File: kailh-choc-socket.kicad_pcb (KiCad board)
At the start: 2 copper layers, 18 x 17 mm, 8 parts, among them SW1 SW_DIP_x01

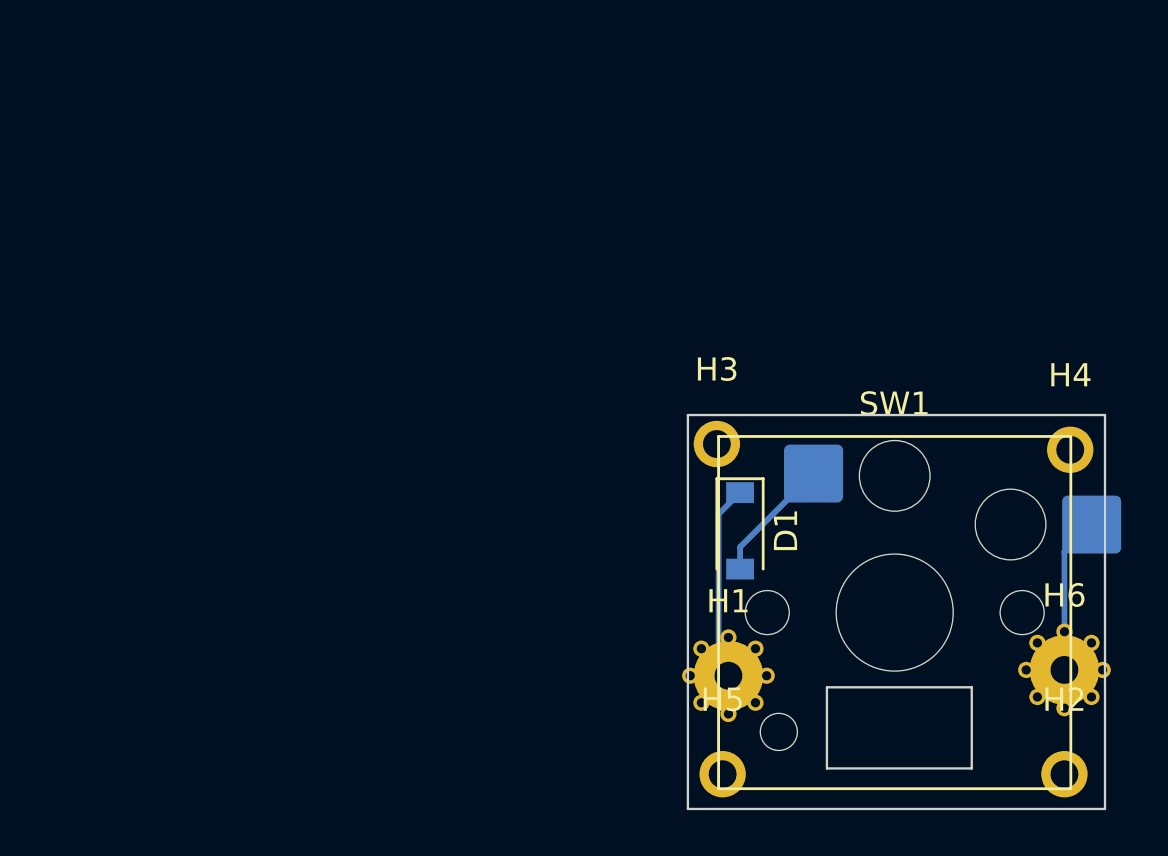
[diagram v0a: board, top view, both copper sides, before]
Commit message: Added layer details
M  .gitignore
M  README.md
M  fp-lib-table
M  kailh-choc-socket.kicad_pcb
M  kailh-choc-socket.kicad_prl
M  kailh-choc-socket.kicad_pro
M  kailh-choc-socket.kicad_sch
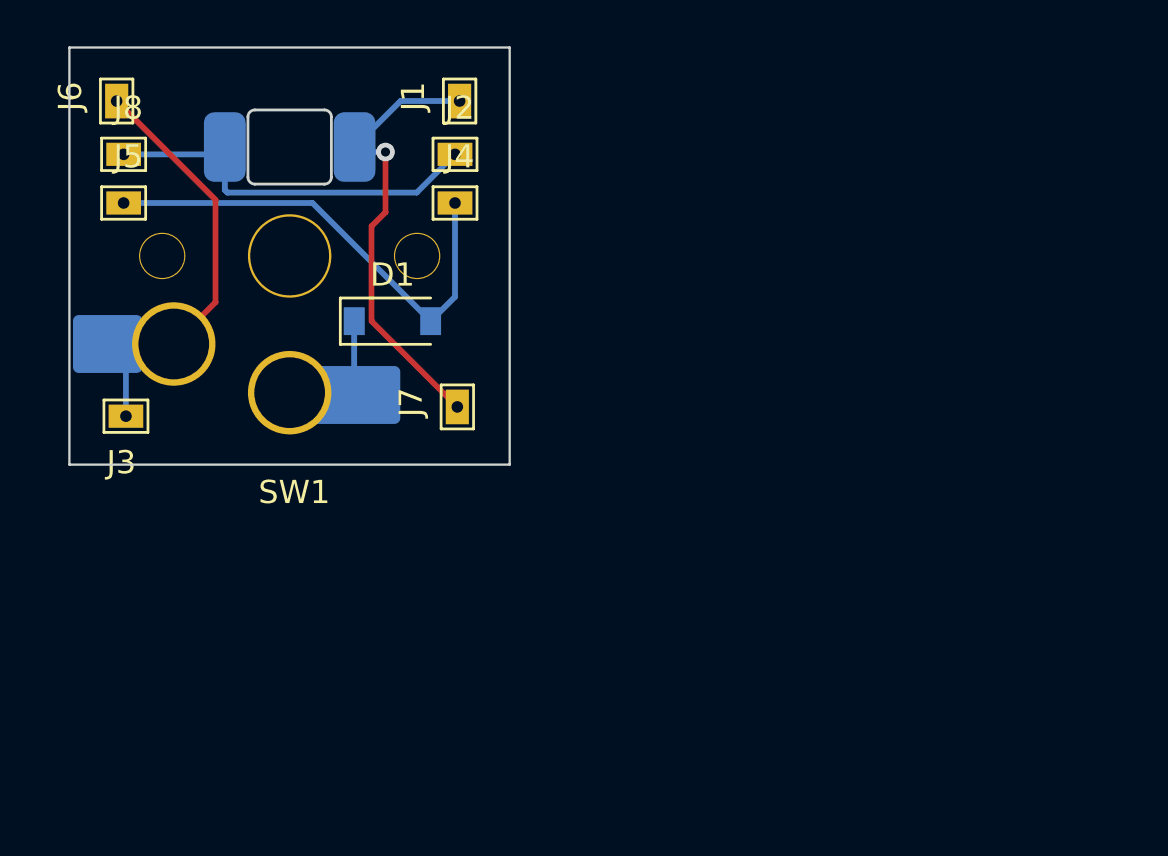
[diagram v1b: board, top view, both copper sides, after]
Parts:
- removed H1, H6: MountingHole_Pad, MountingHole:MountingHole_2.2mm_M2_Pad_Via
- removed H2, H3, H4, H5: MountingHole, MountingHole:MountingHole_2mm
- added J1: Conn_01x01_Male, Giri-Kailh-Choc-Library:TestPoint_THTPad_1.0x1.5mm_Drill0.5mm, F.Cu at (126.4, 69.2)
- added J2: Conn_01x01_Male, Giri-Kailh-Choc-Library:TestPoint_THTPad_1.0x1.5mm_Drill0.5mm, F.Cu at (126.2, 71.5)
- added J3: Conn_01x01_Male, Giri-Kailh-Choc-Library:TestPoint_THTPad_1.0x1.5mm_Drill0.5mm, F.Cu at (112.0, 82.8)
- added J4: Conn_01x01_Male, Giri-Kailh-Choc-Library:TestPoint_THTPad_1.0x1.5mm_Drill0.5mm, F.Cu at (126.2, 73.6)
- added J5: Conn_01x01_Male, Giri-Kailh-Choc-Library:TestPoint_THTPad_1.0x1.5mm_Drill0.5mm, F.Cu at (111.9, 73.6)
- added J6: Conn_01x01_Male, Giri-Kailh-Choc-Library:TestPoint_THTPad_1.0x1.5mm_Drill0.5mm, F.Cu at (111.6, 69.2)
- added J7: Conn_01x01_Male, Giri-Kailh-Choc-Library:TestPoint_THTPad_1.0x1.5mm_Drill0.5mm, F.Cu at (126.3, 82.4)
- added J8: Conn_01x01_Male, Giri-Kailh-Choc-Library:TestPoint_THTPad_1.0x1.5mm_Drill0.5mm, F.Cu at (111.9, 71.5)
- SW1: value SW_DIP_x01 -> SW_DIP_x02; footprint Switch_Keyboard_Hotswap_Kailh:SW_Hotswap_Kailh_Choc_V1_1.00u -> Giri-Kailh-Choc-Library:SW_Hotswap_Kailh_Choc_V1_plated_girish2
- moved SW1 30.3 mm to (119.1, 75.9)
- moved D1 17.5 mm to (123.5, 78.7), turned to 0 degrees
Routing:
- net Net-(J6-Pad1): track 0.00 -> 17.4 mm
- net Net-(J2-Pad1): track 0.00 -> 17.0 mm
- net Net-(J1-Pad1): track 6.76 -> 19.6 mm, vias 0 -> 1
- net Net-(J4-Pad1): track 8.46 -> 20.9 mm
- net Net-(D1-Pad1): track 5.44 -> 3.21 mm
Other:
- board size 18 x 17 mm -> 19 x 18 mm
- board text added: "AmoebaChoc (1.2mm PCB)"
- board text added: "Girish"
- board text added: "Kailh Choc Hotswap"
- board text added: "SMD 6028 Monochorome LED"
- board text added: "SOD-123 Diode"
